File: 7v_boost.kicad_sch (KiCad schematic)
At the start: 5 parts, among them U401 LM27313XMFX/NOPB

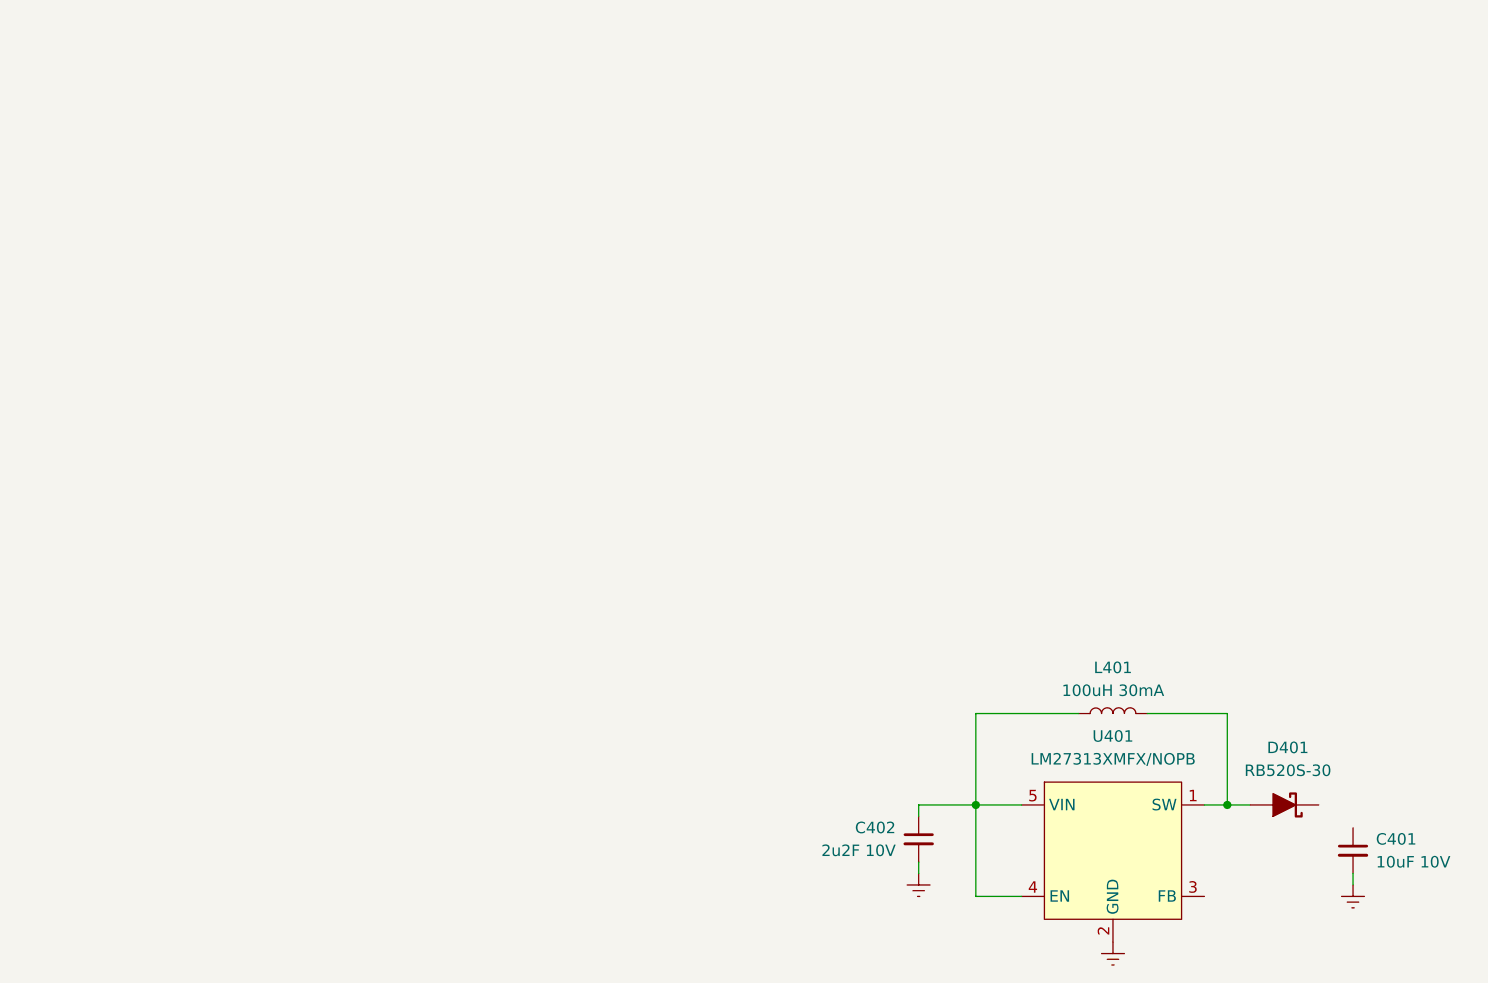
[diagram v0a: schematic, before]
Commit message: Update 7v_boost.kicad_sch
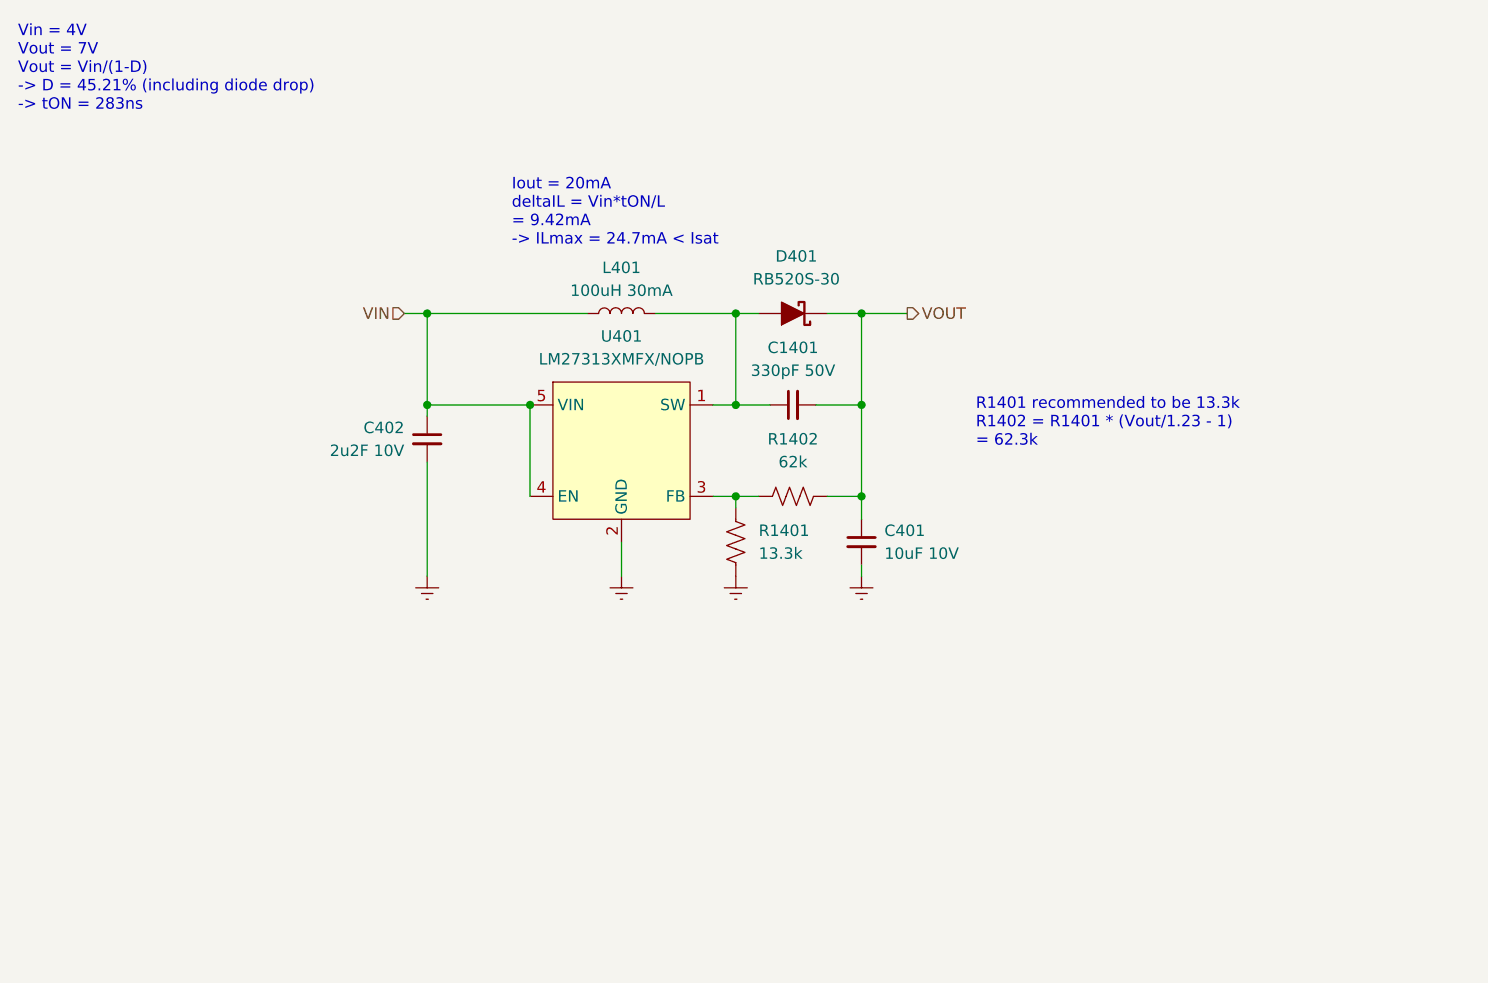
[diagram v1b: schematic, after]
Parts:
- added C1401: 330pF 50V, BR_Passives:C_0402_1005Metric, symbol BR_Capacitors_0402:C_0402_330pF_50V_C0G_5%
- added R1401: 13.3k, BR_Passives:C_0402_1005Metric-minimized, symbol BR_Resistors_0402:R_0402_13k3
- added R1402: 62k, BR_Passives:C_0402_1005Metric-minimized, symbol BR_Resistors_0402:R_0402_62k
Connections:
- net GND: now also R1401.2
- net VIN: now reaches C402.1, L401.1, U401.4 (EN), U401.5 (VIN)
- net at D401.2 (A), L401.2, U401.1 (SW): now also C1401.1
- net VOUT: now reaches C401.1
- net VOUT: now also D401.1 (K), C1401.2, R1402.2
- net at U401.3 (FB): now also R1401.1, R1402.1
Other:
- note added: "Iout = 20mA deltaIL = Vin*tON/L = 9.42mA -> ILmax = 24.7mA < Isat"
- note added: "R1401 recommended to be 13.3k R1402 = R1401 * (Vout/1.23 - 1) = 62.3k"
- note added: "Vin = 4V Vout = 7V Vout = Vin/(1-D) -> D = 45.21% (including diode drop) -> tON = 283ns"
- moved on the sheet: C401, C402, D401, L401, U401
